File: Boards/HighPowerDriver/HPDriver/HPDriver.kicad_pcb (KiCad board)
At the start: 4 copper layers, 107 parts, among them J1 USB_B_Mini, J2 60V_In, J3 Coils, J4 Screw_Terminal_01x06, J5 AVR-ISP-6, Q1 IRFR5410, Q10 IRF4950S, Q11 BC817, Q12 BC817, Q13 BC817, Q14 BC817, Q2 IRFR3910, Q3 IRFR3910, Q4 IRFR5410, Q5 IRFR5410, Q6 IRFR3910, Q7 IRFR3910, Q8 IRFR5410, Q9 BC817, SW1 SW_Push, U1 LM5009MM, U10 ATtiny2313A-SU, U2 TMC262, U3 FT230XS, U4 SFH6156, U5 SFH6156, U6 TLP118, U7 LTV-827S, U8 LTV-827S, U9 74HC14, X1 16MHz, Y1 20MHz

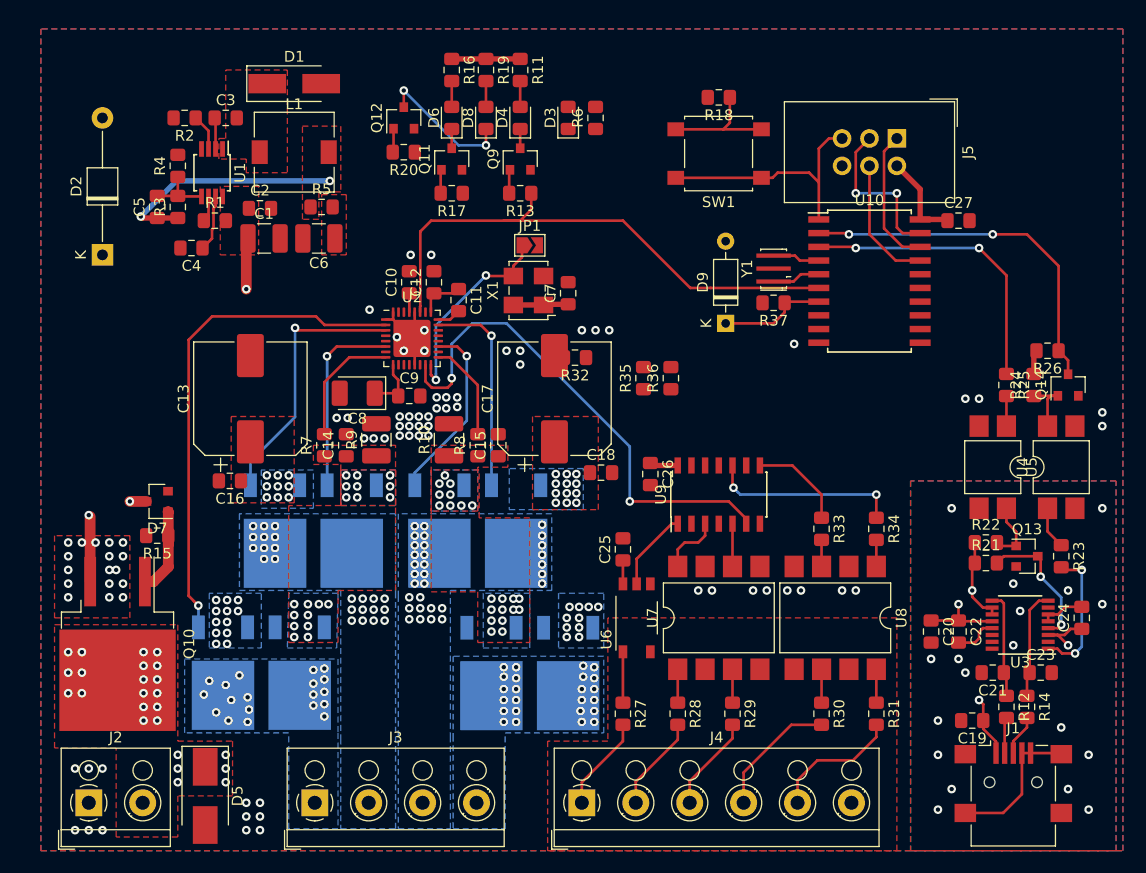
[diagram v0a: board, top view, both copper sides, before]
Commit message: Updated Layout
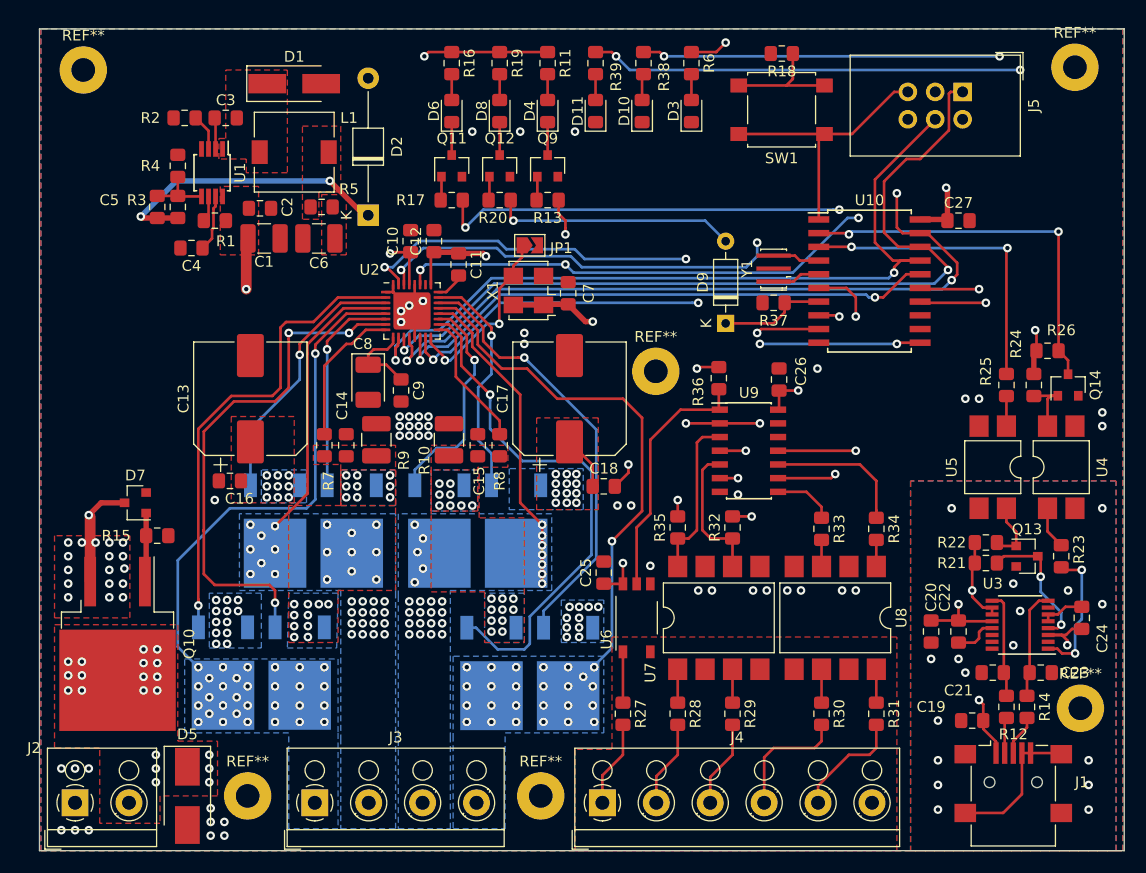
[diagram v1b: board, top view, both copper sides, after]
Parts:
- added D10: LED_Gn, LED_SMD:LED_0805_2012Metric_Pad1.15x1.40mm_HandSolder, F.Cu at (140.2, 72.4)
- added D11: LED_Rt, LED_SMD:LED_0805_2012Metric_Pad1.15x1.40mm_HandSolder, F.Cu at (135.9, 72.4)
- added R38: 180R, Resistor_SMD:R_0805_2012Metric_Pad1.15x1.40mm_HandSolder, F.Cu at (140.3, 67.9)
- added R39: 180R, Resistor_SMD:R_0805_2012Metric_Pad1.15x1.40mm_HandSolder, F.Cu at (135.9, 67.9)
- added REF**: MountingHole_2.2mm_M2_Pad, MountingHole:MountingHole_2.2mm_M2_Pad, F.Cu at (180.3, 68.3)
- added REF**: MountingHole_2.2mm_M2_Pad, MountingHole:MountingHole_2.2mm_M2_Pad, F.Cu at (88.4, 68.6)
- added REF**: MountingHole_2.2mm_M2_Pad, MountingHole:MountingHole_2.2mm_M2_Pad, F.Cu at (141.5, 96.5)
- added REF**: MountingHole_2.2mm_M2_Pad, MountingHole:MountingHole_2.2mm_M2_Pad, F.Cu at (180.8, 127.8)
- added REF**: MountingHole_2.2mm_M2_Pad, MountingHole:MountingHole_2.2mm_M2_Pad, F.Cu at (130.8, 135.9)
- added REF**: MountingHole_2.2mm_M2_Pad, MountingHole:MountingHole_2.2mm_M2_Pad, F.Cu at (103.6, 135.9)
- moved D2 24.9 mm to (114.8, 82.0)
- moved R32 21.5 mm to (148.6, 111.0), turned to 90 degrees
- moved C26 14.8 mm to (152.9, 97.3), turned to 90 degrees
- moved R35 14.2 mm to (143.5, 111.0)
- moved D3 11.4 mm to (144.8, 72.4)
- moved R6 10.2 mm to (144.8, 67.9), turned to 270 degrees
- moved Q12 9.94 mm to (127.0, 77.5)
- moved R20 9.94 mm to (127.0, 80.6)
- moved J5 7.47 mm to (169.9, 70.6)
- moved R18 7.12 mm to (153.2, 67.1)
- moved SW1 7.12 mm to (153.1, 72.3)
- moved U9 4.93 mm to (150.1, 103.9), turned to 0 degrees
- moved R36 4.44 mm to (147.3, 97.2)
- moved C10 3.81 mm to (118.7, 84.5)
- moved C12 3.81 mm to (120.9, 84.5)
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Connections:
- U10 pad 14: (no net) -> /Connector/Error
- U10 pad 15: (no net) -> /Connector/Active
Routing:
- net /Connector/Step: track 0.00 -> 76.3 mm, vias 0 -> 6
- net /Connector/Ready: track 0.00 -> 70.1 mm, vias 0 -> 4
- net /Connector/Error: track 0.00 -> 69.1 mm, vias 0 -> 3
- net /Controller/MISO: track 12.9 -> 79.7 mm, vias 0 -> 2
- net /Connector/Dir: track 0.00 -> 65.8 mm, vias 0 -> 4
- net /Controller/SCK: track 15.0 -> 78.9 mm, vias 2 -> 3
- net /Controller/MOSI: track 12.1 -> 74.4 mm, vias 0 -> 2
- net /Connector/Active: track 0.00 -> 61.1 mm, vias 0 -> 3
- net /Controller/CS_TMC: track 0.00 -> 52.3 mm, vias 0 -> 2
- net /Connector/Coil_A1: track 0.00 -> 51.4 mm, vias 19 -> 31
- net /Connector/Coil_B2: track 0.00 -> 50.2 mm, vias 24 -> 26
- net Net-(Q3-Pad1): track 0.00 -> 48.5 mm, vias 0 -> 1
- net Net-(Q6-Pad1): track 0.00 -> 47.9 mm, vias 0 -> 3
- net Net-(Q4-Pad1): track 0.00 -> 40.7 mm, vias 0 -> 1
- net /Connector/Stall: track 51.9 -> 86.2 mm, vias 0 -> 6
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- added copper zone on In1.Cu, net +5V
- added copper zone on In1.Cu, net GNDS
- added copper zone on In2.Cu, net GNDS
- removed copper zone on In1.Cu, net GND
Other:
- board outline added: 100.6 x 76.2 mm
